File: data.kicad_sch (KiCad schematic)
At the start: 29 parts, among them J2 GSB4D313302Y1HR, U11 FT601Q, U12 HD3SS3220, U13 ABM8-30.000MHZ-D1X-T

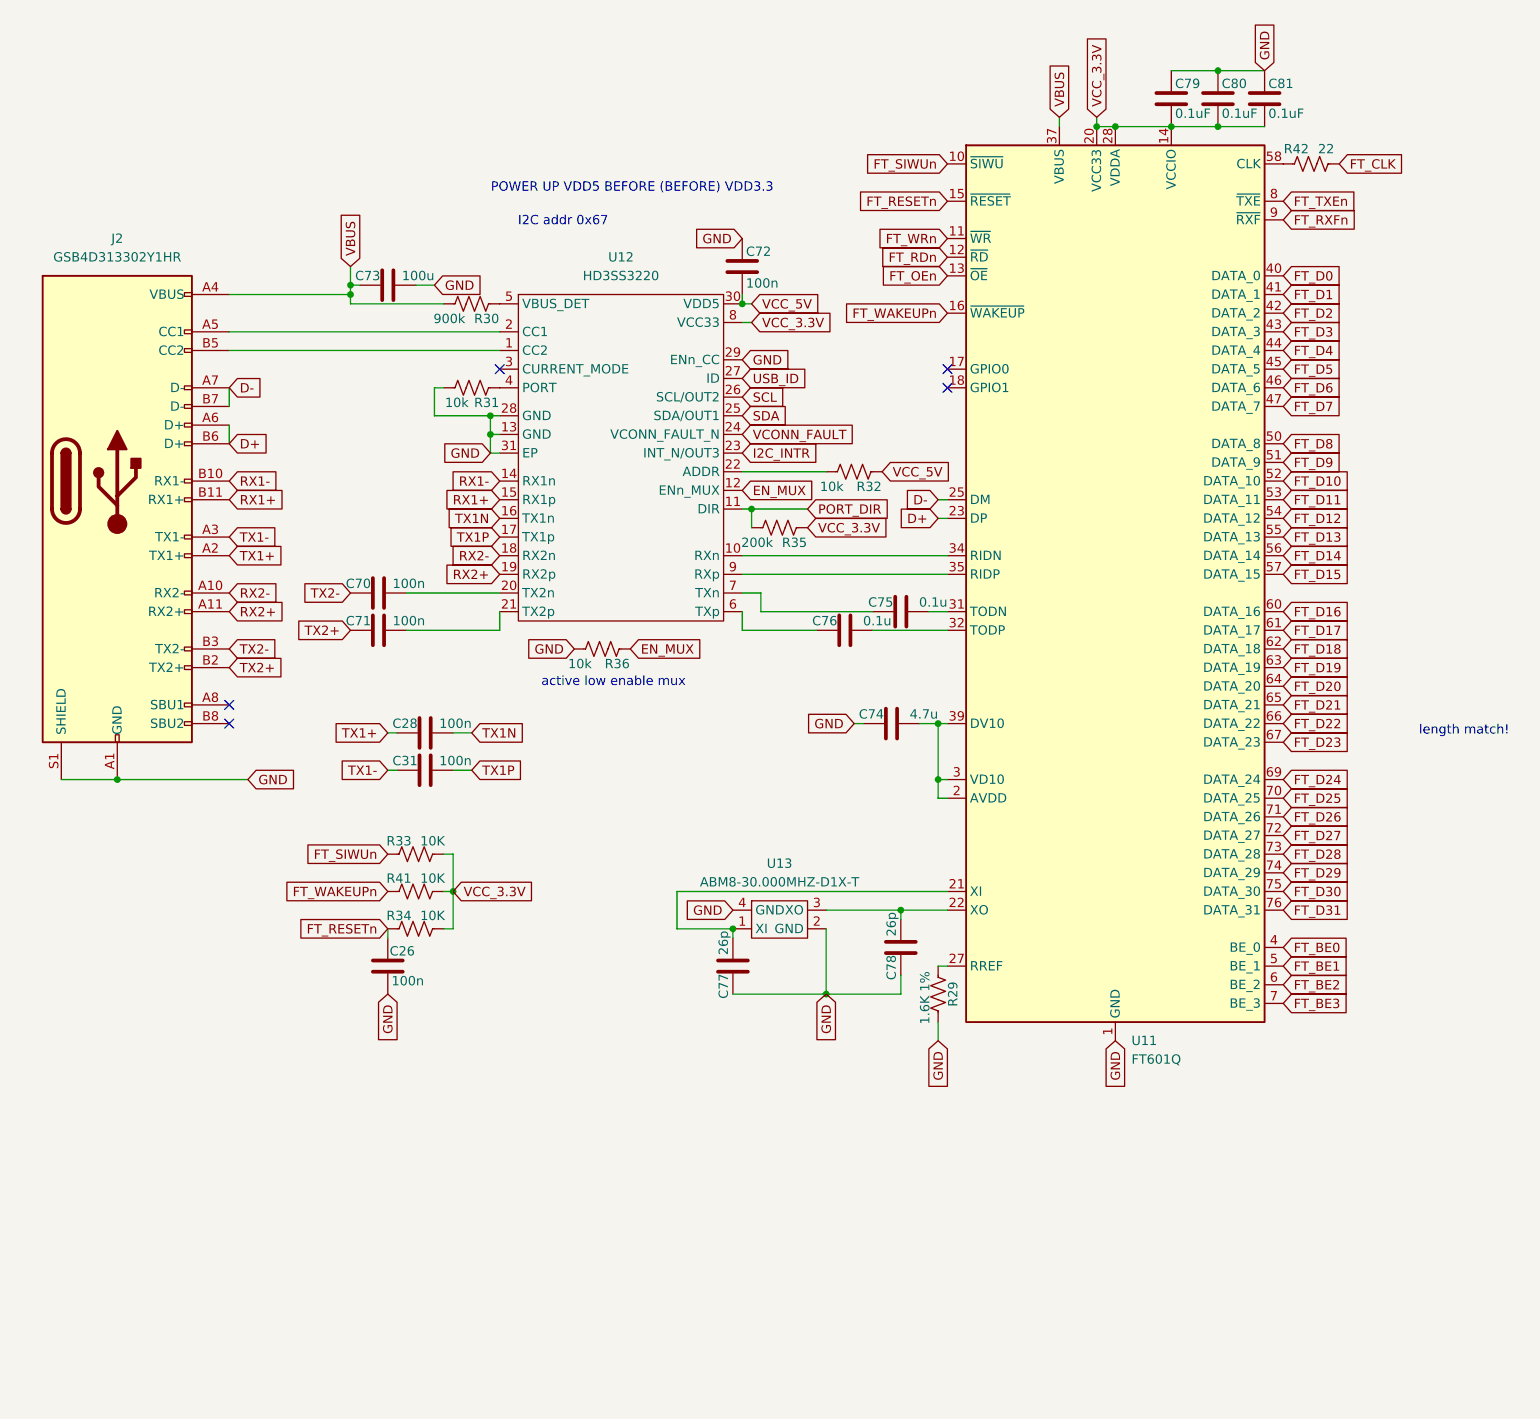
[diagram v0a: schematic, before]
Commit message: some moderate pcb work
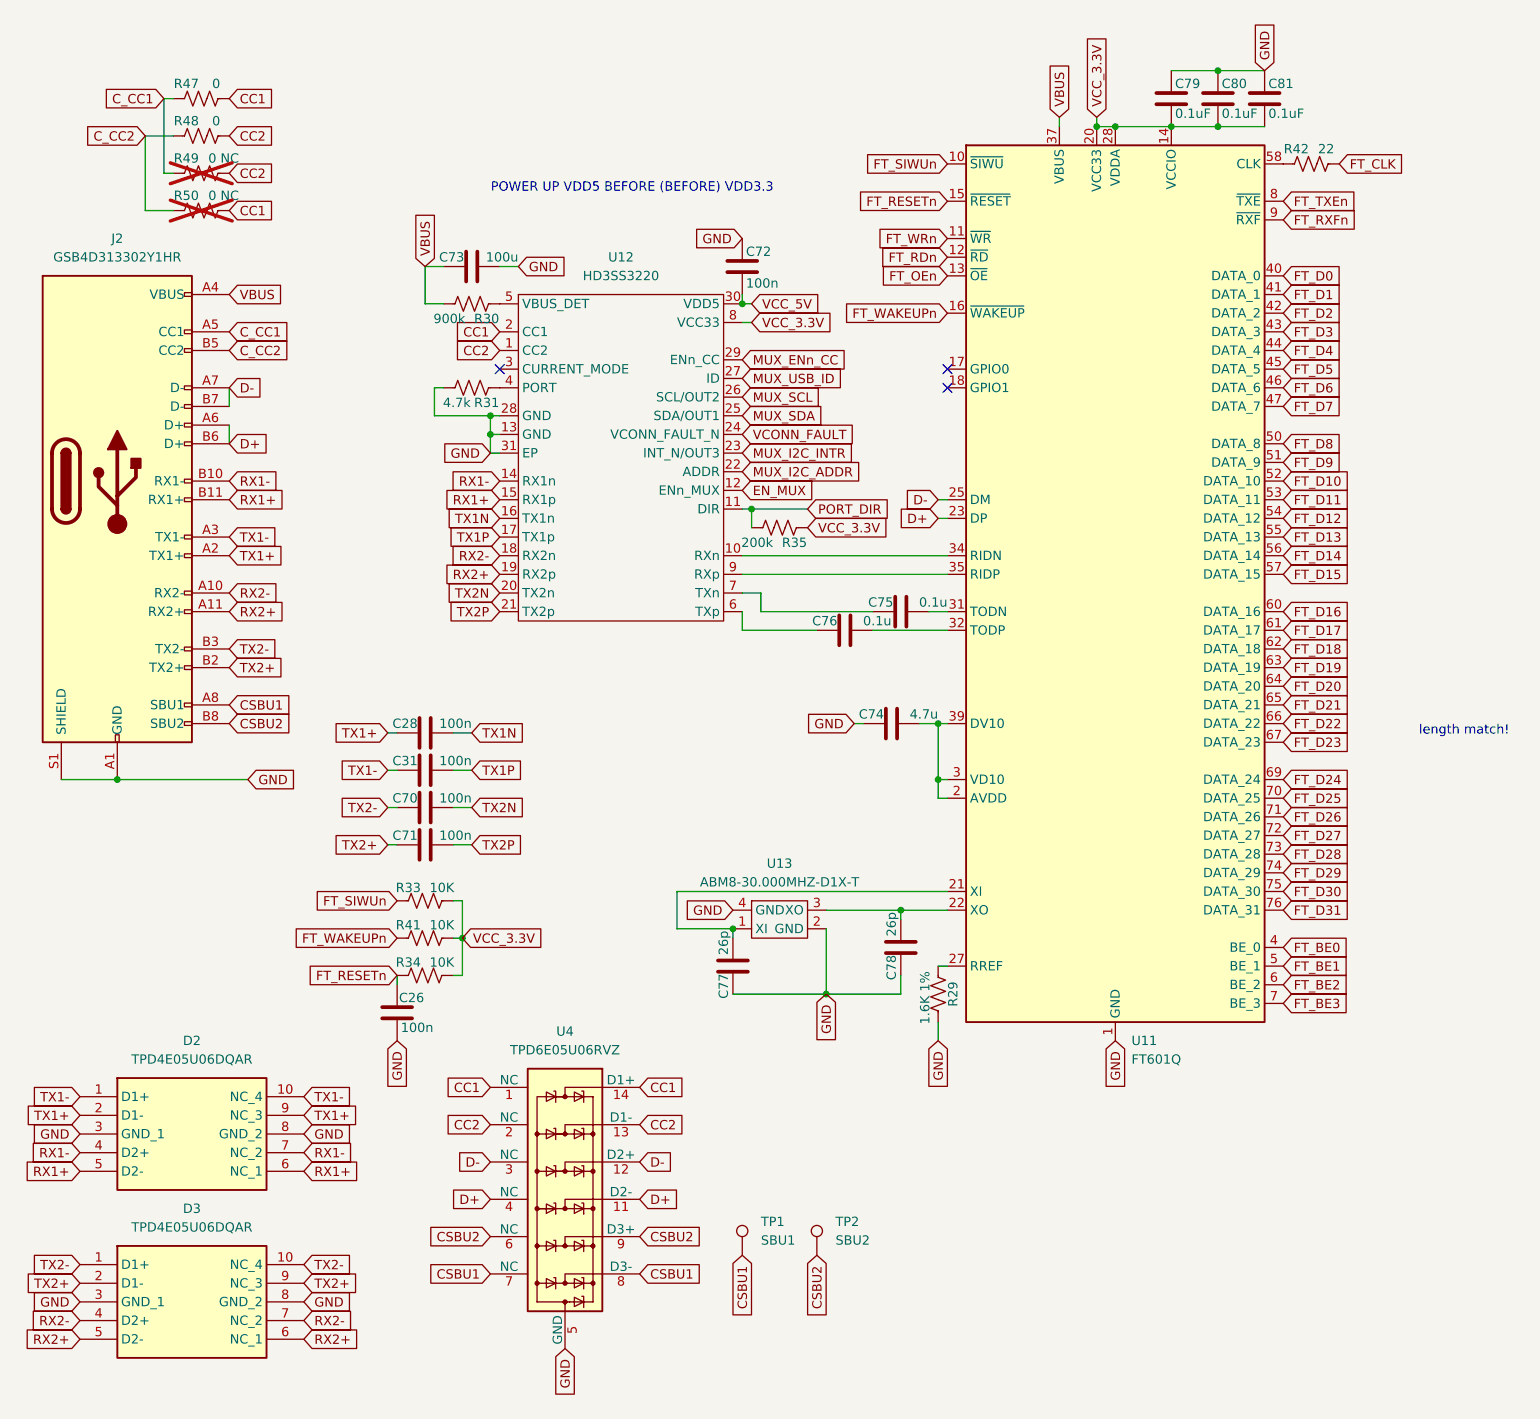
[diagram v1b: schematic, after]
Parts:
- removed R32, R36: 10k, Resistor_SMD:R_0402_1005Metric, symbol Device:R_US
- added D2, D3: TPD4E05U06DQAR, hfsdr:SON50P135X350X55-14N, symbol hfsdr:TPD4E05U06DQAR
- added R47, R48: 0, Resistor_SMD:R_0402_1005Metric, symbol Device:R_US
- added R49, R50: 0 NC, Resistor_SMD:R_0402_1005Metric, symbol Device:R_US
- added TP1: SBU1, TestPoint:TestPoint_Pad_D1.0mm, symbol Connector:TestPoint
- added TP2: SBU2, TestPoint:TestPoint_Pad_D1.0mm, symbol Connector:TestPoint
- added U4: TPD6E05U06RVZ, Package_SON:Texas_R-PUSON-N14, symbol Power_Protection:TPD6E05U06RVZ
- R31: value 10k -> 4.7k
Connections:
- net D+: now also U4.11 (D2-), U4.4 (NC)
- net D-: now also U4.12 (D2+), U4.3 (NC)
- net GND: now also D2.3 (GND_1), D2.8 (GND_2), D3.3 (GND_1), D3.8 (GND_2), U4.10 (GND), U4.5 (GND); no longer U12.29 (ENn_CC)
- net RX1+: now also D2.5 (D2-), D2.6 (NC_1)
- net RX1-: now also D2.4 (D2+), D2.7 (NC_2)
- net RX2+: now also D3.5 (D2-), D3.6 (NC_1)
- net RX2-: now also D3.4 (D2+), D3.7 (NC_2)
- net TX1+: now also D2.2 (D1-), D2.9 (NC_3)
- net TX1-: now also D2.1 (D1+), D2.10 (NC_4)
- net TX2+: now also D3.2 (D1-), D3.9 (NC_3)
- net TX2-: now also D3.1 (D1+), D3.10 (NC_4)
- net CC1: now reaches U12.2 (CC1)
- net CC1: now also R47.2, R50.2, U4.1 (NC), U4.14 (D1+); no longer J2.A5 (CC1)
- net CSBU1: now reaches J2.A8 (SBU1)
- net CSBU1: now also TP1.1, U4.7 (NC), U4.8 (D3-)
- net CC2: now reaches U12.1 (CC2)
- net CC2: now also R48.2, R49.2, U4.13 (D1-), U4.2 (NC); no longer J2.B5 (CC2)
- net CSBU2: now reaches J2.B8 (SBU2)
- net CSBU2: now also TP2.1, U4.6 (NC), U4.9 (D3+)
- net TX2N: now reaches C70.2, U12.20 (TX2n)
- net TX2P: now reaches C71.2, U12.21 (TX2p)
- net MUX_I2C_ADDR: now reaches U12.22 (ADDR)
- net I2C_INTR renamed MUX_I2C_INTR
- net SCL renamed MUX_SCL
- net SDA renamed MUX_SDA
- net USB_ID renamed MUX_USB_ID
- new net C_CC1: J2.A5 (CC1), R47.1, R49.1
- new net C_CC2: J2.B5 (CC2), R48.1, R50.1
- new net MUX_ENn_CC: U12.29 (ENn_CC)
- no-connect marks 5 -> 3
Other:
- note removed: "I2C addr 0x67"
- note removed: "active low enable mux"
- moved on the sheet: C26, C73, R33, R34, R41
